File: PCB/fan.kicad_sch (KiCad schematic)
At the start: 12 parts, among them M1 P8 Max, U10 TMP468xxRGT, U11 LP5907MFX-3.3

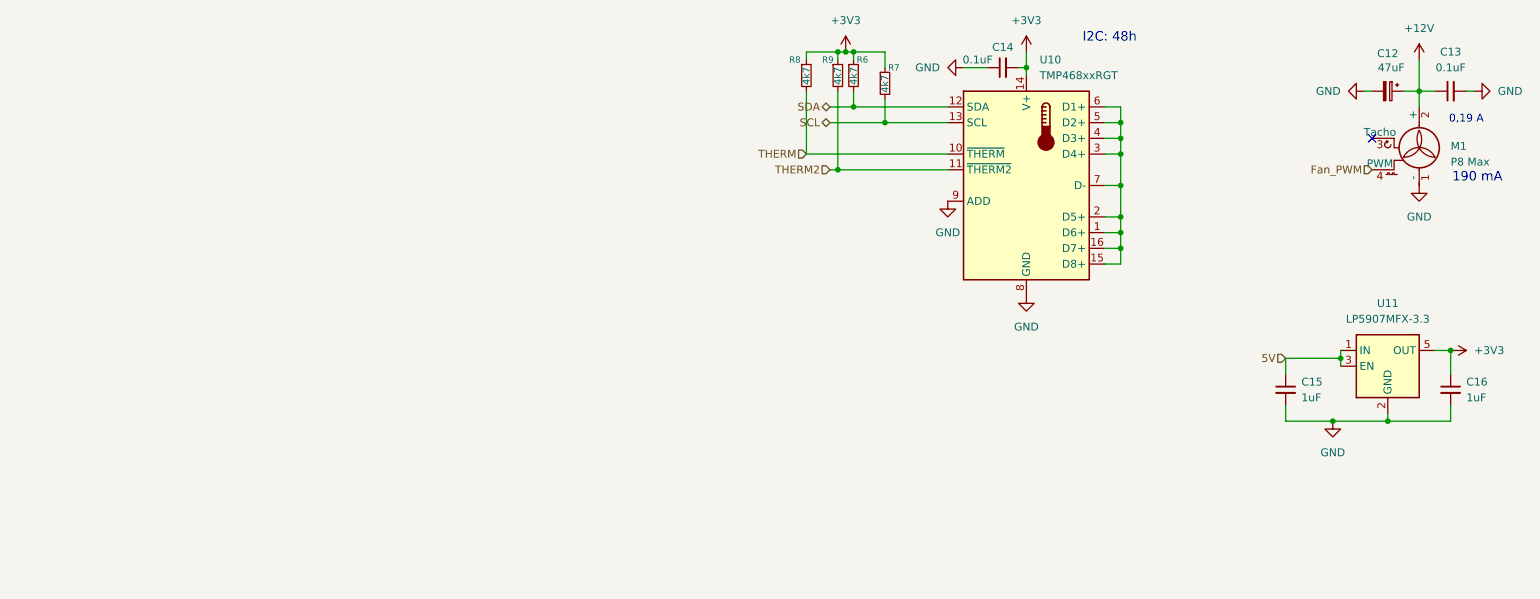
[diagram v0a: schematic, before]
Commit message: Initial commit of project source code
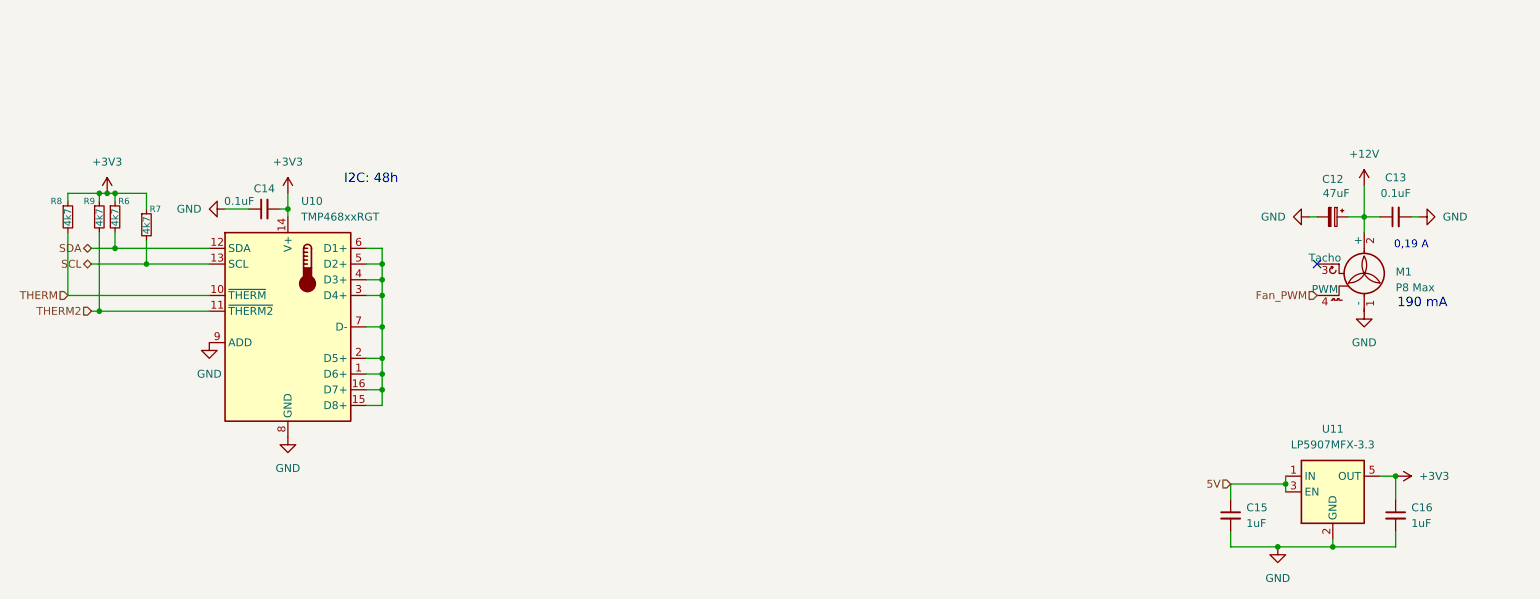
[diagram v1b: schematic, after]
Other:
- moved on the sheet: C12, C13, C14, C15, C16, M1, R6, R7, R8, R9, U10, U11
